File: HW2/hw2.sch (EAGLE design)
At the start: 7 parts, among them J2 USB_

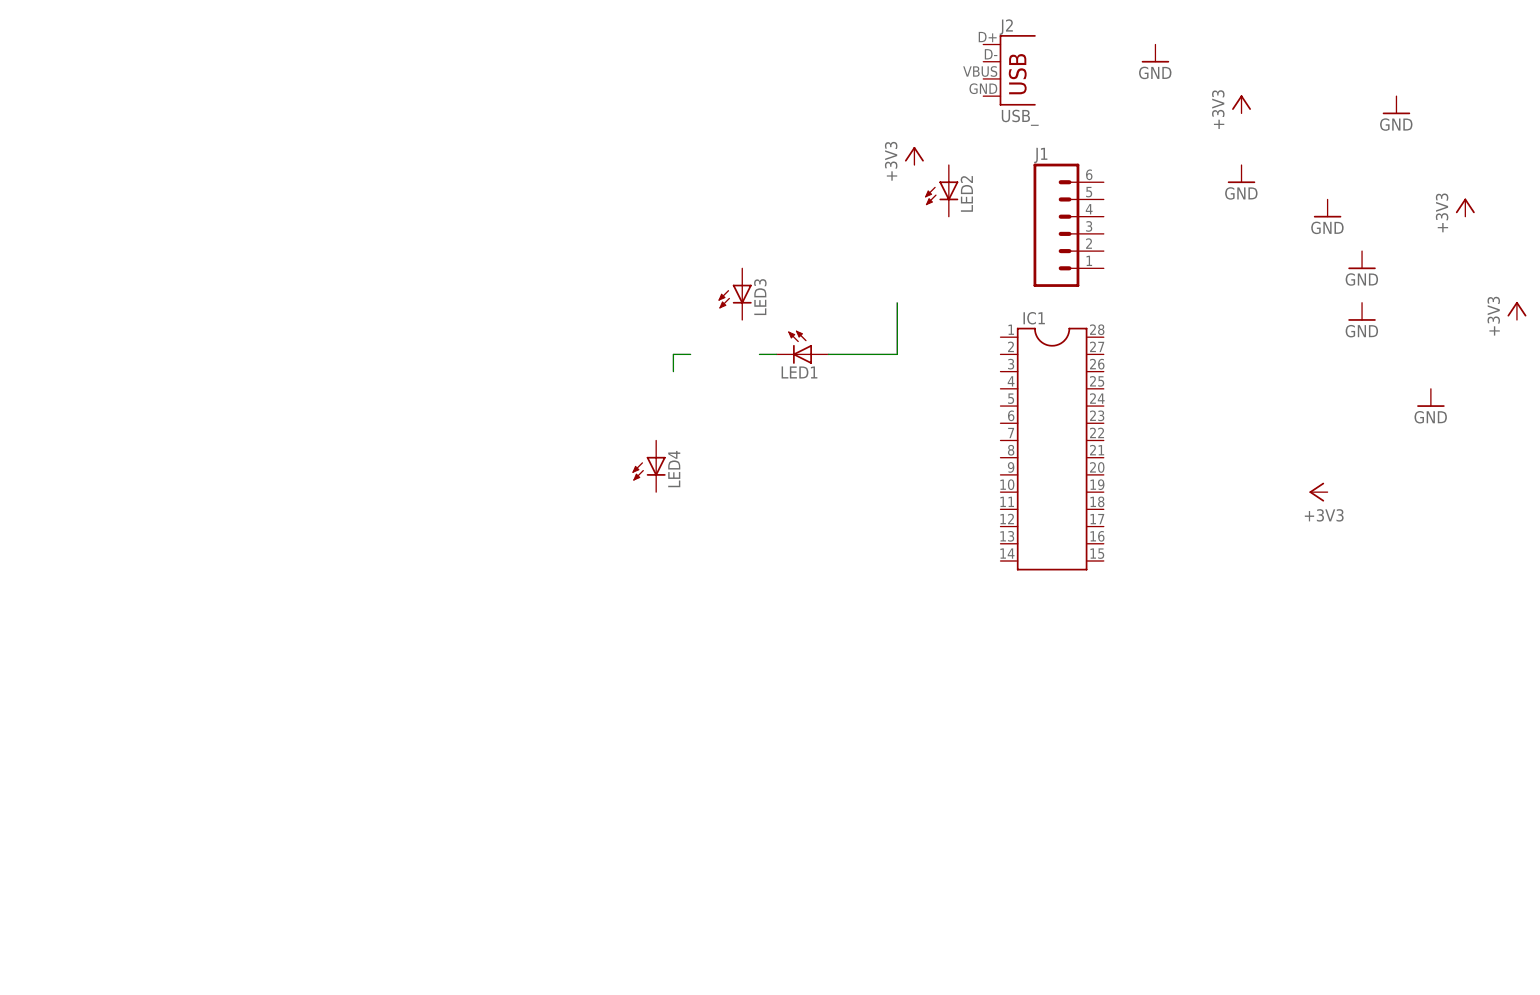
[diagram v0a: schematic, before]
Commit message: Ready to be checked before order
Ready to be checked before order
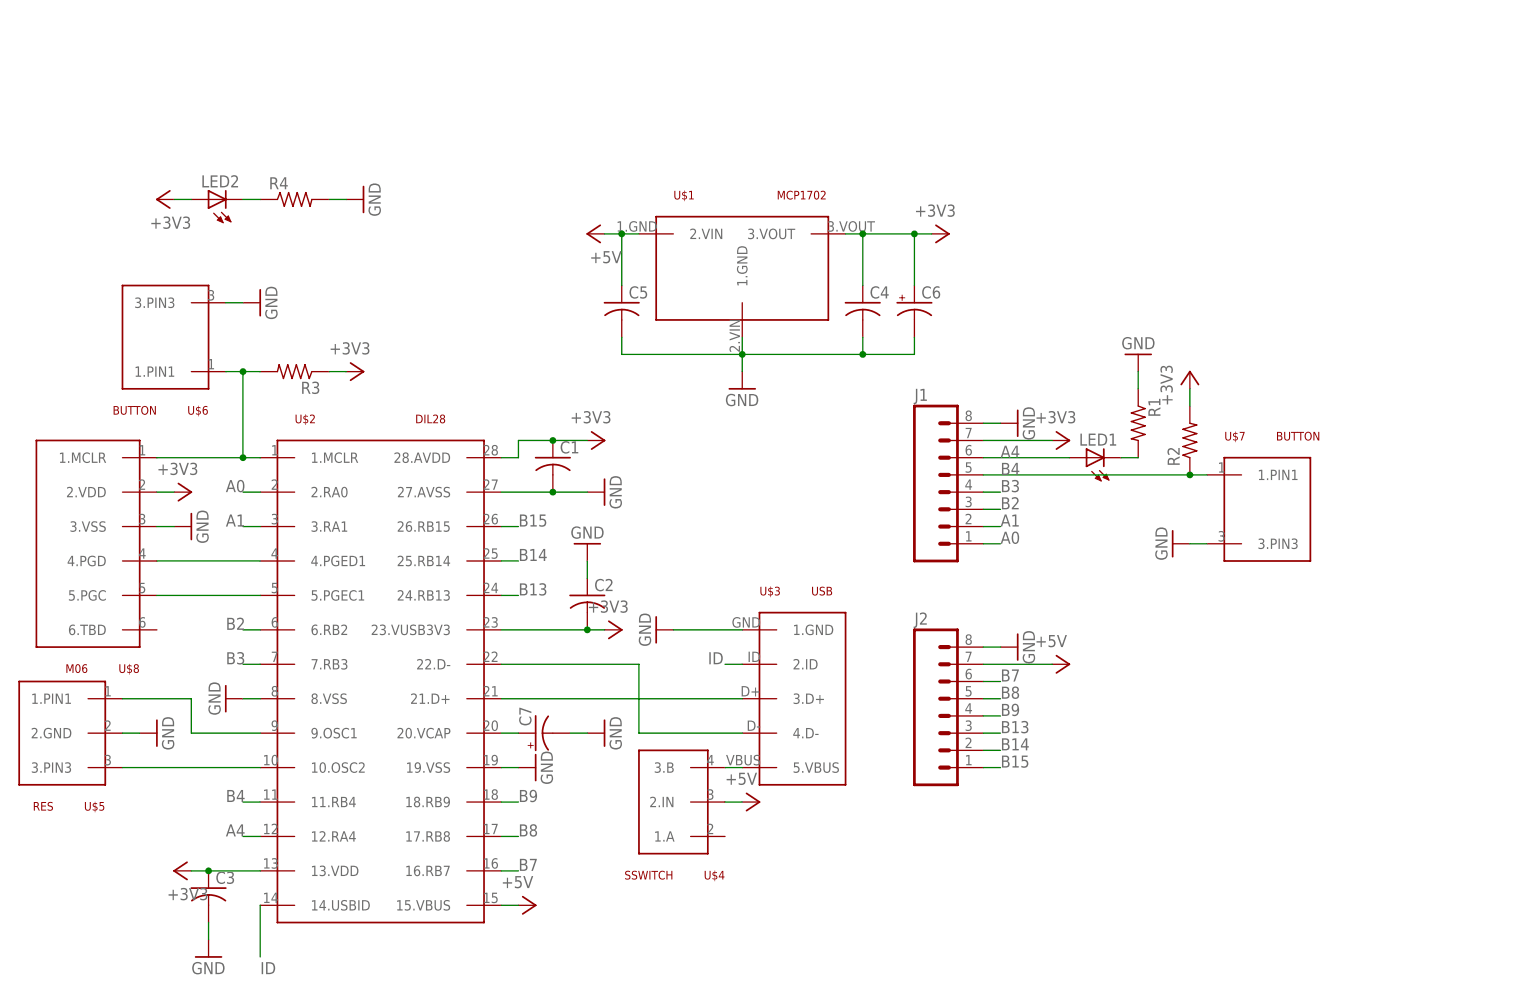
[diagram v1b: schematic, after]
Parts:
- removed IC1: (no value), hw2:DIL28-3
- removed LED3, LED4: (no value), led:LED3MM
- added C1, C2, C3, C4, C5: (no value), hw2:C-US025-025X050
- added C6, C7: (no value), hw2:CPOL-USTT2D4L
- added R1, R2, R3, R4: (no value), hw2:R-US_0207/10
- added U$1: MCP1702, hw2:MCP1702
- added U$2: DIL28, hw2:DIL28
- added U$3: USB, hw2:USB
- added U$4: SSWITCH, hw2:SSWITCH
- added U$5: RES, hw2:RES
- added U$6, U$7: BUTTON, hw2:BUTTON
- added U$8: M06, hw2:M06
- J1: device hw2:M06SILK_FEMALE_PTH -> hw2:M08
- J2: value USB_ -> (none); device hw2:USB_ -> hw2:M08
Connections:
- new net +3V3: C1.1, C2.2, C3.1, C4.1, C6.+, J1.7, LED2.A, R2.2, R3.1, U$1.3.VOUT, U$2.13.VDD, U$2.23.VUSB3V3, U$2.28.AVDD, U$8.2.VDD
- new net +5V: C5.1, J2.7, U$1.2.VIN, U$2.15.VBUS, U$4.2.IN
- new net A0: J1.1, U$2.2.RA0
- new net A1: J1.2, U$2.3.RA1
- new net A4: J1.6, LED1.A, U$2.12.RA4
- new net B13: J2.3, U$2.24.RB13
- new net B14: J2.2, U$2.25.RB14
- new net B15: J2.1, U$2.26.RB15
- new net B2: J1.3, U$2.6.RB2
- new net B3: J1.4, U$2.7.RB3
- new net B4: J1.5, R2.1, U$2.11.RB4, U$7.1.PIN1
- new net B7: J2.6, U$2.16.RB7
- new net B8: J2.5, U$2.17.RB8
- new net B9: J2.4, U$2.18.RB9
- new net GND: C1.2, C2.1, C3.2, C4.2, C5.2, C6.-, C7.-, J1.8, J2.8, R1.1, R4.2, U$1.1.GND, U$2.19.VSS, U$2.27.AVSS, U$2.8.VSS, U$3.1.GND, U$5.2.GND, U$6.3.PIN3, U$7.3.PIN3, U$8.3.VSS
- new net ID: U$2.14.USBID, U$3.2.ID
- new net N$11: U$3.5.VBUS, U$4.3.B
- new net N$12: U$2.21.D+, U$3.3.D+
- new net N$13: U$2.22.D-, U$3.4.D-
- new net N$2: LED2.C, R4.1
- new net N$4: U$2.10.OSC2, U$5.3.PIN3
- new net N$5: C7.+, U$2.20.VCAP
- new net N$7: U$2.5.PGEC1, U$8.5.PGC
- new net N$8: U$2.4.PGED1, U$8.4.PGD
- new net N$9: R3.2, U$2.1.MCLR, U$6.1.PIN1, U$8.1.MCLR
- net N$1: now also LED1.C, R1.2; no longer LED1.A
- net N$3: now also U$2.9.OSC1, U$5.1.PIN1; no longer LED1.C
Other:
- moved on the sheet: LED1, LED2
